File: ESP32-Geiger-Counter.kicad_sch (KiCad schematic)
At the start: 42 parts, among them J1 2s1p Lipo Battery Pack (8.4V-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, J2 USB_C_Receptacle_USB2.0_16P, SW1 SW_SPDT, SW2 RESET, SW3 BOOT, U1 BQ25886RGE, U2 AP63203WU, U3 ESP32-S3-WROOM-1

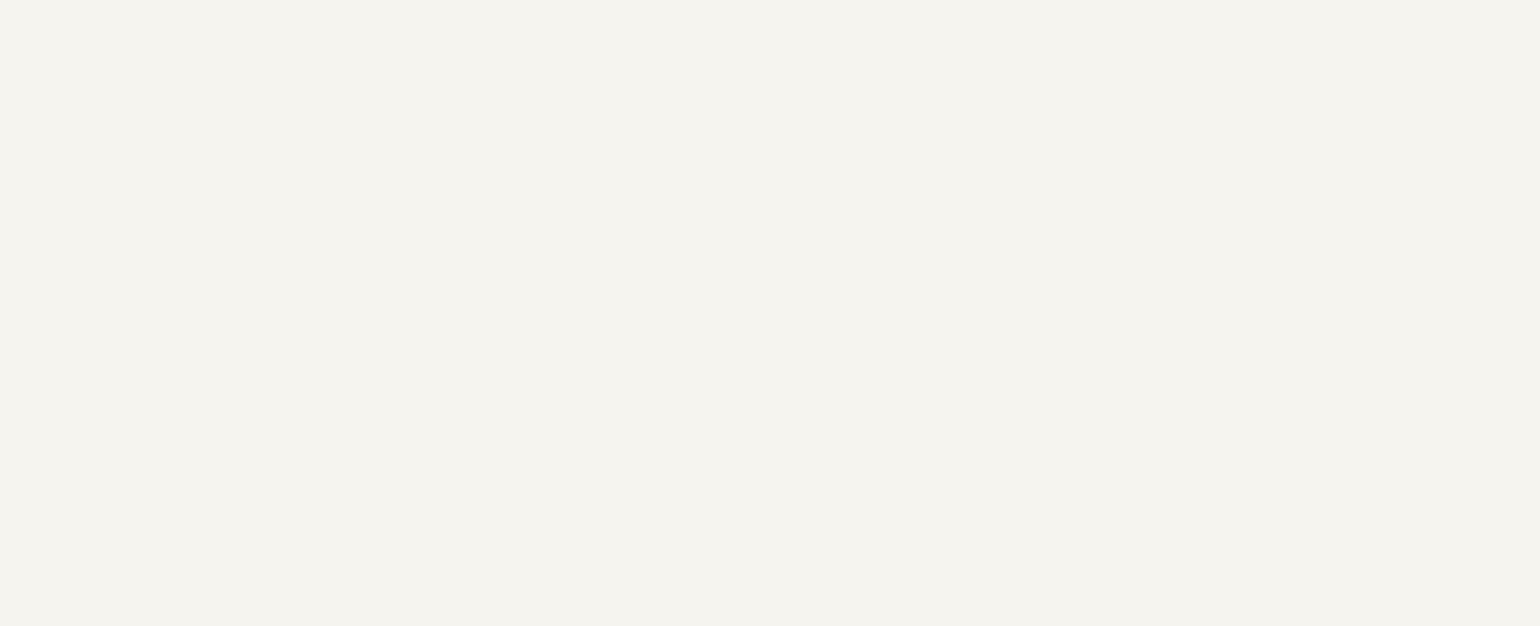
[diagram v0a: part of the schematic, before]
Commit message: working on HV boost
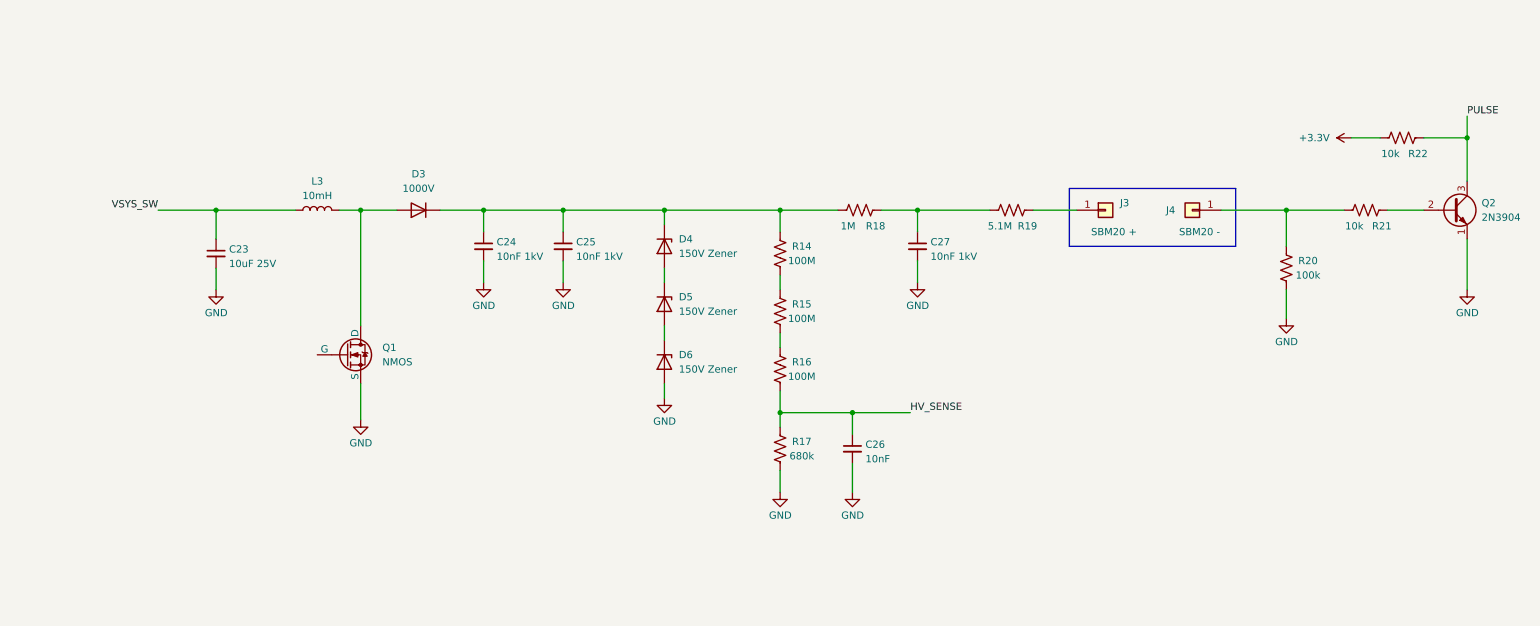
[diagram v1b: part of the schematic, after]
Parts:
- added C23: 10uF 25V, symbol Device:C_Small
- added C24, C25, C27: 10nF 1kV, symbol Device:C_Small
- added C26: 10nF, symbol Device:C_Small
- added D3: 1000V, symbol Device:D
- added D4, D5, D6: 150V Zener, symbol Device:D_Zener
- added J3: SBM20 +, symbol Connector_Generic:Conn_01x01
- added J4: SBM20 -, symbol Connector_Generic:Conn_01x01
- added L3: 10mH, symbol Device:L
- added Q1: NMOS, symbol Simulation_SPICE:NMOS
- added Q2: 2N3904, Package_TO_SOT_THT:TO-92_Inline, symbol Transistor_BJT:2N3904
- added R14, R15, R16: 100M, symbol Device:R_US
- added R17: 680k, symbol Device:R_US
- added R18: 1M, symbol Device:R_US
- added R19: 5.1M, symbol Device:R_US
- added R20: 100k, symbol Device:R_US
- added R21, R22: 10k, symbol Device:R_US
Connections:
- net +3.3V: now also R22.1
- net GND: now also C23.2, C24.2, C25.2, C26.2, C27.2, D6.2 (A), Q1.3 (S), Q2.1 (E), R17.1, R20.1
- net VSYS_SW: now also C23.1, L3.1
- new net: J4.1 (Pin_1), R20.2, R21.1
- new net: C24.1, C25.1, D3.1 (K), D4.1 (K), R14.2, R18.1
- new net: D3.2 (A), L3.2, Q1.1 (D)
- new net: R15.1, R16.2
- new net: R14.1, R15.2
- new net: D4.2 (A), D5.1 (K)
- new net: D5.2 (A), D6.1 (K)
- new net: C27.1, R18.2, R19.1
- new net: J3.1 (Pin_1), R19.2
- new net: Q2.2 (B), R21.2
- new net HV_SENSE: C26.1, R16.1, R17.2
- new net PULSE: Q2.3 (C), R22.2
